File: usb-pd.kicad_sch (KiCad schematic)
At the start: 0 parts

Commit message: workin on the schematic
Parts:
- added C1, C2: 1uF, symbol Device:C
- added C3: 0.1uF, symbol Device:C
- added J1: USB_C_Receptacle_PowerOnly_6P, symbol Connector:USB_C_Receptacle_PowerOnly_6P
- added J2: USB3_A, Connector_USB:USB3_A_Molex_48406-0001_Horizontal_Stacked, symbol Connector:USB3_A
- added U1: CYPD3177-24LQ, Package_DFN_QFN:QFN-24-1EP_4x4mm_P0.5mm_EP2.75x2.75mm, symbol Interface_USB:CYPD3177-24LQ
- added U2: AMS1117-3.3, Package_TO_SOT_SMD:SOT-223-3_TabPin2, symbol Regulator_Linear:AMS1117-3.3
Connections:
- new net: C3.1, U1.11 (VDC_OUT)
- new net +3.3V: C2.2, U1.23 (VDDD), U1.24 (VCCD), U2.2 (VO)
- new net CC1: J1.A5 (CC1), U1.15 (CC1)
- new net CC2: J1.B5 (CC2), U1.14 (CC2)
- new net GND: C1.1, C2.1, C3.2, J1.A12 (GND), J1.B12 (GND), J1.S1 (SHIELD), J2.10 (SHIELD), J2.4 (GND), J2.7 (DRAIN), U1.1 (VBUS_MIN), U1.19 (GND), U1.22 (GND), U1.25 (GND), U1.5 (ISNK_COARSE), U1.6 (ISNK_FINE), U2.1 (GND)
- new net VBUS: C1.2, J2.1 (VBUS), U2.3 (VI)
- new net VBUS_C: J1.A9 (VBUS), J1.B9 (VBUS), U1.18 (VBUS_IN)
- no-connect marks 0 -> 6
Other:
- note added: "PD Negotionations"
- note added: "USB Input"
- note added: "USB Output"

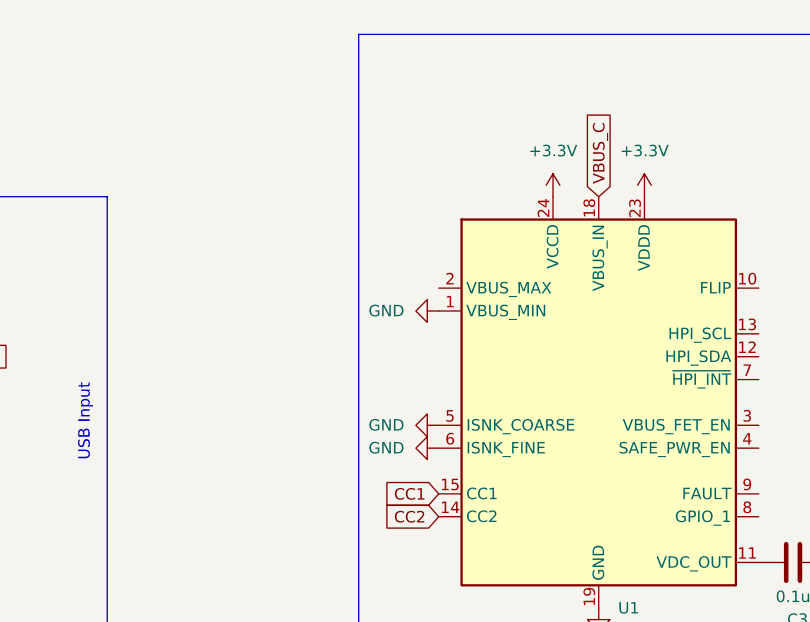
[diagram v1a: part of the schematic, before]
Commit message: trying to work on the PD IC some more
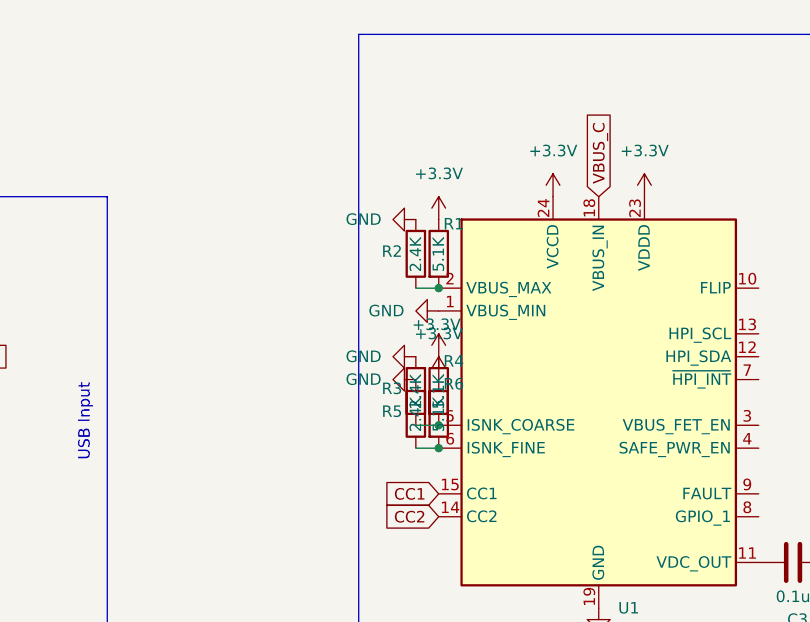
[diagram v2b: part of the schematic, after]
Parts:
- added R1, R4, R6: 5.1K, symbol Device:R
- added R2, R3, R5: 2.4K, symbol Device:R
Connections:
- net +3.3V: now also R1.1, R4.1, R6.1
- net GND: now also R2.2, R3.2, R5.2; no longer U1.5 (ISNK_COARSE), U1.6 (ISNK_FINE)
- net at U1.2 (VBUS_MAX): now also R1.2, R2.1
- new net: R5.1, R6.2, U1.6 (ISNK_FINE)
- new net: R3.1, R4.2, U1.5 (ISNK_COARSE)
